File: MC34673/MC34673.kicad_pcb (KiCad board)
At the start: 2 copper layers, 44.2 x 21.3 mm, 12 parts, among them J1 dc_jack, M1 MC34673, P1 CONN_01X02

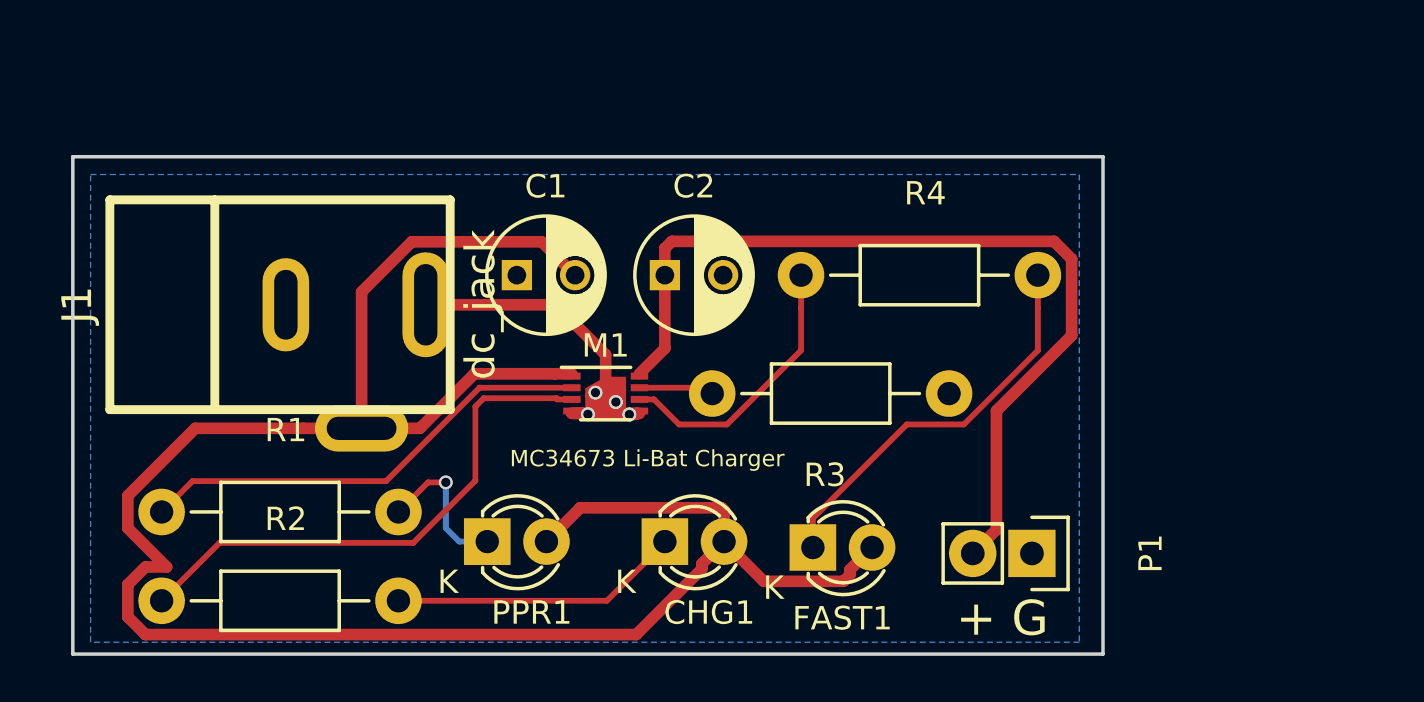
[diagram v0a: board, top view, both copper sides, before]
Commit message: ready for ickey
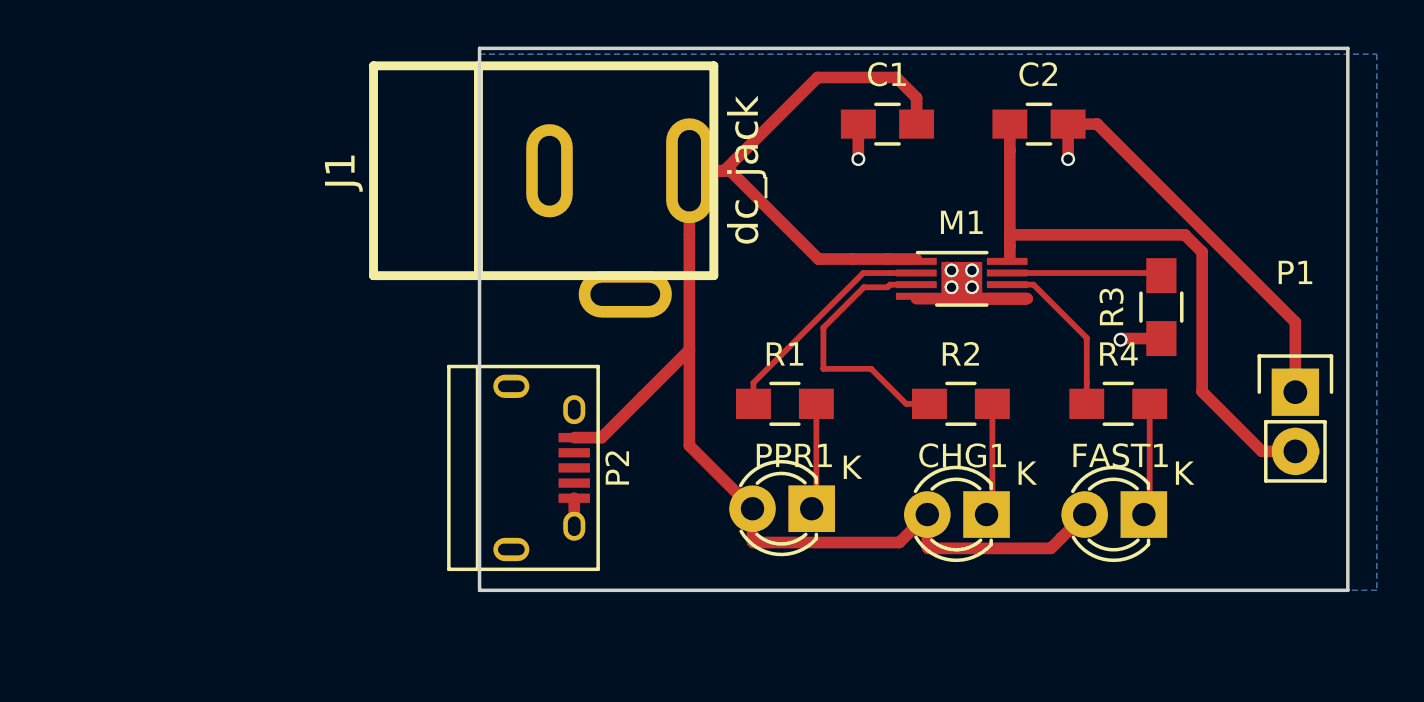
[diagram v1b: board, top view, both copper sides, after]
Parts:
- added P2: USB_OTG, Connect:USB_Micro-B, F.Cu at (134.2, 102.2)
- C1, C2: footprint Capacitors_ThroughHole:C_Radial_D5_L11_P2.5 -> Capacitors_SMD:C_0805_HandSoldering
- R1, R2, R3, R4: footprint Resistors_ThroughHole:Resistor_Horizontal_RM10mm -> Resistors_SMD:R_0805_HandSoldering
- moved R2 35.3 mm to (152.4, 99.5)
- moved R1 27.1 mm to (144.8, 99.5)
- moved C2 17.3 mm to (155.8, 87.5)
- moved C1 17.2 mm to (149.2, 87.5)
- moved M1 16.1 mm to (152.4, 94.1)
- moved R4 14.7 mm to (159.1, 99.5)
- moved FAST1 14.3 mm to (160.2, 104.2), turned to 180 degrees
- moved PPR1 14.0 mm to (146.0, 104.0), turned to 180 degrees
- moved CHG1 13.8 mm to (153.5, 104.2), turned to 180 degrees
- moved P1 13.3 mm to (166.8, 99.0), turned to 0 degrees
- moved J1 12.7 mm to (134.5, 89.5)
- moved R3 9.83 mm to (161.0, 95.3), turned to 90 degrees
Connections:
- J1 pad 1: +5V -> Net-(J1-Pad1)
- J1 pad 2: Net-(J1-Pad2) -> Earth
- J1 pad 3: Earth -> +5V
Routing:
- net +5V: track 89.9 -> 64.5 mm
- net Net-(C2-Pad1): track 38.1 -> 25.6 mm
- net Net-(FAST1-Pad1): track 17.1 -> 4.85 mm
- net Net-(M1-Pad3): track 23.1 -> 11.7 mm
- net Net-(M1-Pad2): track 19.8 -> 9.84 mm
- net Earth: track 22.1 -> 31.4 mm, vias 4 -> 7
- net Net-(CHG1-Pad1): track 12.5 -> 4.85 mm
- net Net-(M1-Pad6): track 11.9 -> 7.19 mm
- net Net-(M1-Pad7): track 3.23 -> 6.66 mm
- net Net-(PPR1-Pad1): track 6.54 -> 4.65 mm, vias 1 -> 0
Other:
- board size 44.2 x 21.3 mm -> 37.2 x 23.2 mm
- board text removed: "+ G"
- board text removed: "MC34673 Li-Bat Charger"
